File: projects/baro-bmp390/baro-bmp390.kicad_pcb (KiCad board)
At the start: 2 copper layers, 18 x 26 mm, 13 parts, among them J1 STEMMA-QT, U1 BMP390

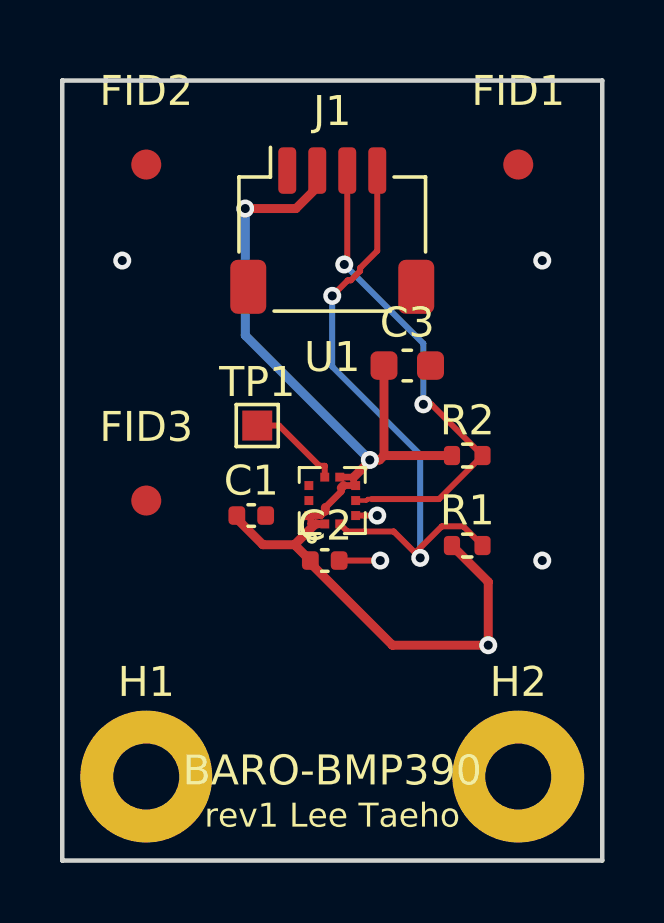
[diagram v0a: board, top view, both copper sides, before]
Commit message: 9/6 update
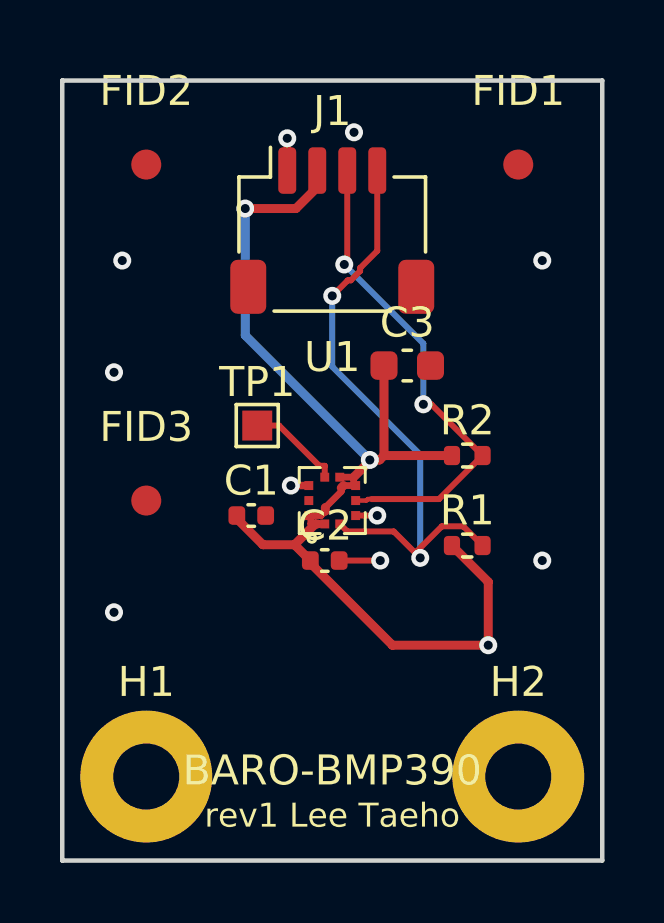
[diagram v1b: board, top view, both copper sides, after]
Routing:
- net GND: track 2.09 -> 3.76 mm, vias 5 -> 10
